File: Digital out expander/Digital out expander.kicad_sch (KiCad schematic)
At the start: 126 parts, among them J1 Screw_Terminal_01x03, J10 Conn_01x03_Pin, J11 Conn_01x03_Pin, J12 Conn_01x03_Pin, J13 Conn_01x03_Pin, J14 Conn_01x03_Pin, J15 Conn_01x03_Pin, J16 Conn_01x03_Pin, J17 Conn_01x03_Pin, J18 Screw_Terminal_01x16, J19 Conn_01x04_Pin, J2 Conn_01x03_Pin, J20 Conn_01x04_Pin, J21 Conn_01x04_Pin, J22 Conn_01x04_Pin, J23 Conn_01x04_Pin, J24 Conn_01x03_Pin, J3 Conn_01x03_Pin, J4 Conn_01x03_Pin, J5 Conn_01x03_Pin, J6 Conn_01x03_Pin, J7 Conn_01x03_Pin, J8 Conn_01x03_Pin, J9 Conn_01x03_Pin, Q1 2N5401, Q10 2N5401, Q11 2N5401, Q12 2N5401, Q13 2N5401, Q14 2N5401, Q15 2N5401, Q16 2N5401, Q17 BC547, Q18 BC547, Q19 BC547, Q2 2N5401, Q20 BC547, Q21 BC547, Q22 BC547, Q23 BC547, Q24 BC547, Q25 BC547, Q26 BC547, Q27 BC547, Q28 BC547, Q29 BC547, Q3 2N5401, Q30 BC547, Q31 BC547, Q32 BC547, Q4 2N5401, Q5 2N5401, Q6 2N5401, Q7 2N5401, Q8 2N5401, Q9 2N5401, U1 PC847, U2 PC847, U3 PC847, U4 PC847, U5 MCP23017_SO

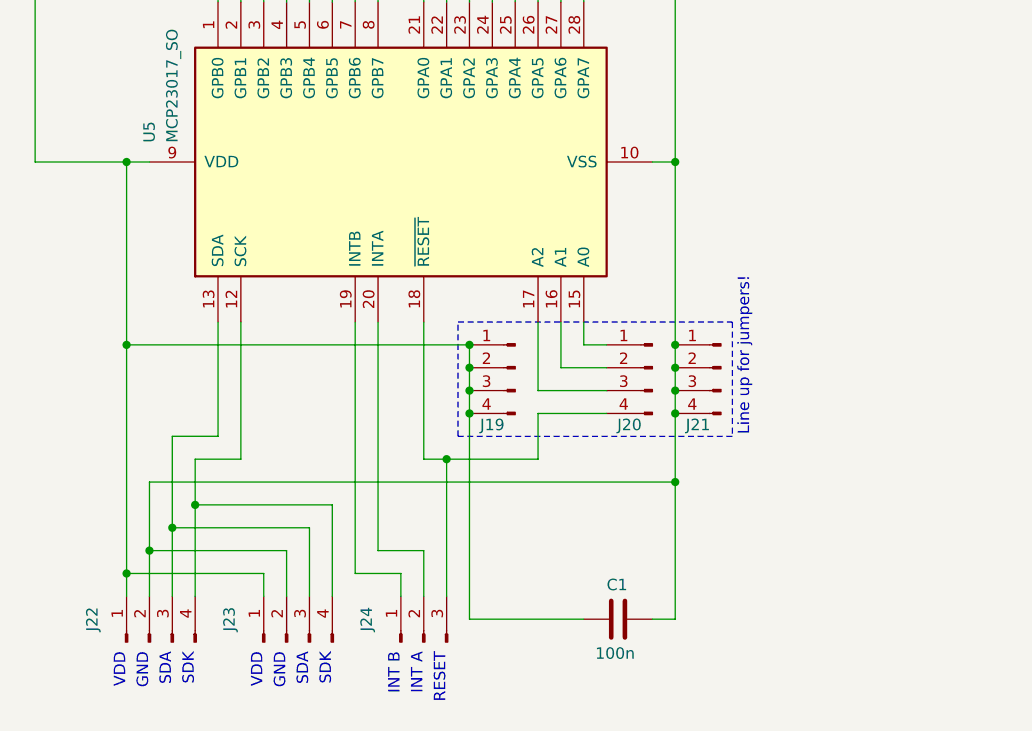
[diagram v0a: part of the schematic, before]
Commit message: Ändrade jumpers för bättre tydlighet
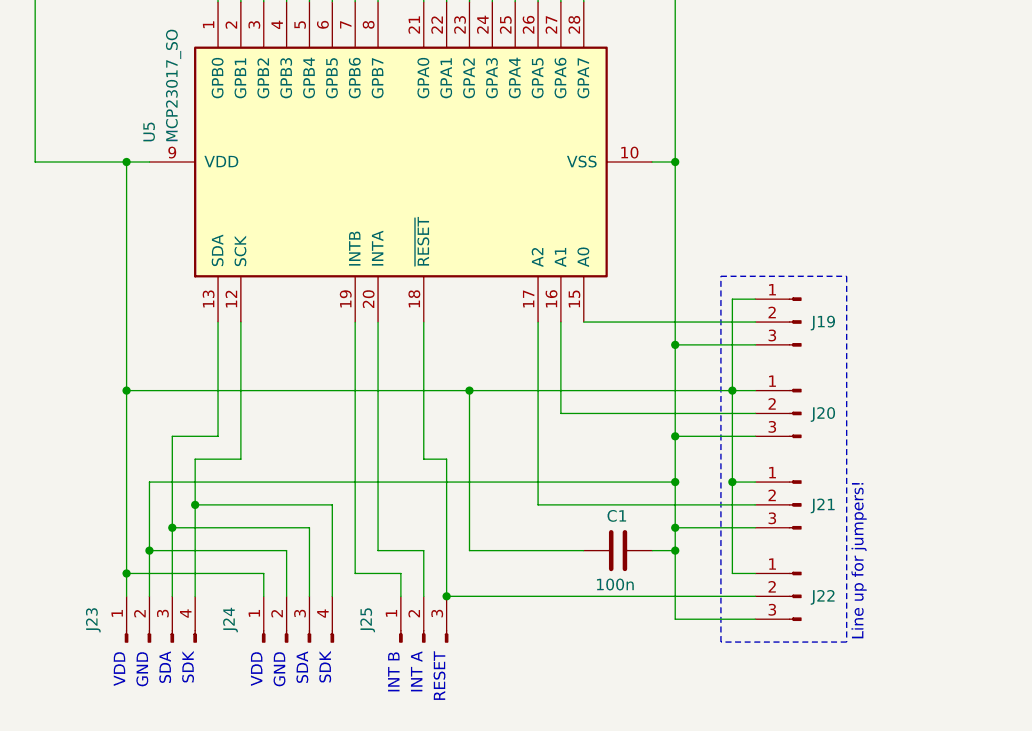
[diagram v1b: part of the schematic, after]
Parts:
- removed J19, J20, J21: Conn_01x04_Pin, symbol Connector:Conn_01x04_Pin
- added J19, J20, J21, J22: Conn_01x03_Pin, symbol Connector:Conn_01x03_Pin
- renumbered J22 to J23, J23 to J24, J24 to J25
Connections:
- net at C1.1, J23.1 (Pin_1), J24.1 (Pin_1)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: now also J19.1 (Pin_1), J20.1 (Pin_1), J21.1 (Pin_1), J22.1 (Pin_1)
- net at C1.2, J23.2 (Pin_2), J24.2 (Pin_2)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: now also J19.3 (Pin_3), J20.3 (Pin_3), J21.3 (Pin_3), J22.3 (Pin_3)
- net at U5.15 (A0): now also J19.2 (Pin_2)
- net at U5.16 (A1): now also J20.2 (Pin_2)
- net at U5.17 (A2): now also J21.2 (Pin_2)
- net at J25.3 (Pin_3), U5.18 (~{RESET}): now also J22.2 (Pin_2)
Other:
- moved on the sheet: C1
